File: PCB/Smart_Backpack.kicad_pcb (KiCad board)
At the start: 2 copper layers, 65.8 x 74.4 mm, 57 parts, among them J1 Conn_01x03_Pin, J2 Conn_01x02_Pin, J3 Conn_01x02_Pin, J4 Conn_01x03_Pin, J5 Conn_01x03_Pin, J6 Conn_01x03_Pin, J7 Conn_01x07_Pin, J8 Conn_01x08_Socket, J9 USB_C_Receptacle_USB2.0_16P, SW1 SW_Push, SW2 SW_Push, U1 TLV62569ADRL, U2 MPU-6050, U3 ESP32-PICO-MINI-02-N8R2, U4 CP2102N-Axx-xQFN28

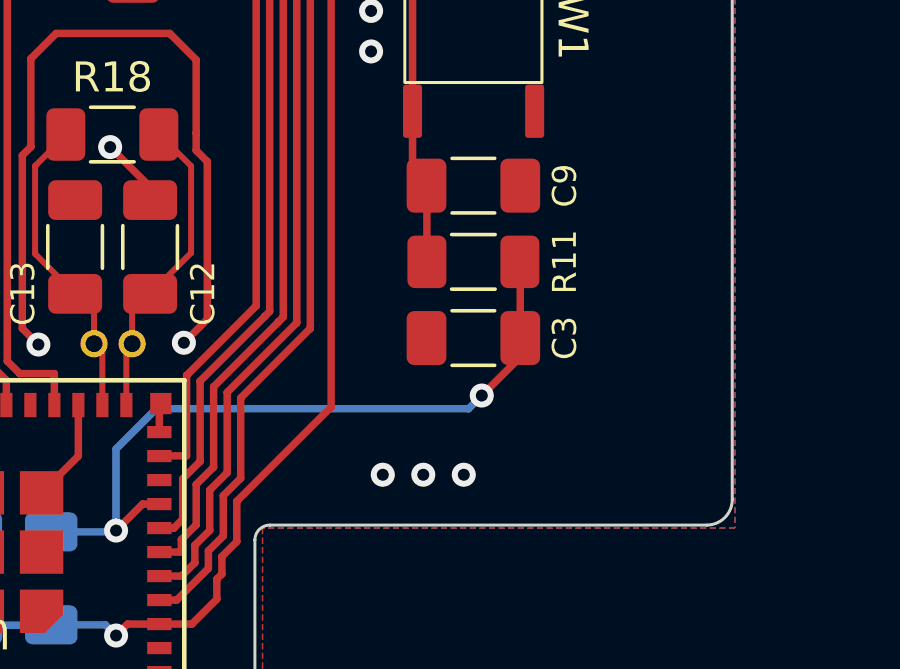
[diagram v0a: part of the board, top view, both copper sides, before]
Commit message: Literally just added our names
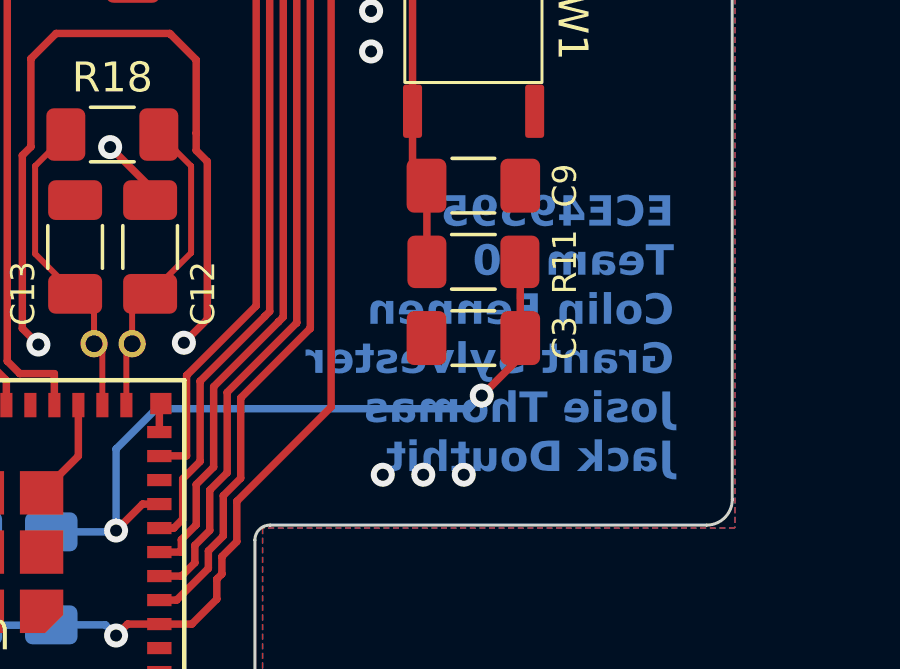
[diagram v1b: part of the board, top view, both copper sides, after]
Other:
- board text added: "ECE49595 Team 10 Colin Fennen Grant Sylvester Josie Thomas Jack Douthit"
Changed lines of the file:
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@@
 		(layer "Edge.Cuts")
+	)
+	(gr_text "ECE49595\nTeam 10\nColin Fennen\nGrant Sylvester\nJosie Thomas\nJack Douthit"
+		(at 149.098 104.14 0)
+		(layer "B.Cu")
+		(effects
+			(font
+				(size 1.016 1.016)
+				(thickness 0.2286)
+				(bold yes)
+			)
+			(justify left bottom mirror)
+		)
 	)
 	(gr_text "+"
